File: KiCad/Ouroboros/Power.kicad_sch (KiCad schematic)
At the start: 8 parts, among them J2 Jack-DC, U1 Opamp_Quad, U3 LM78L05_TO92

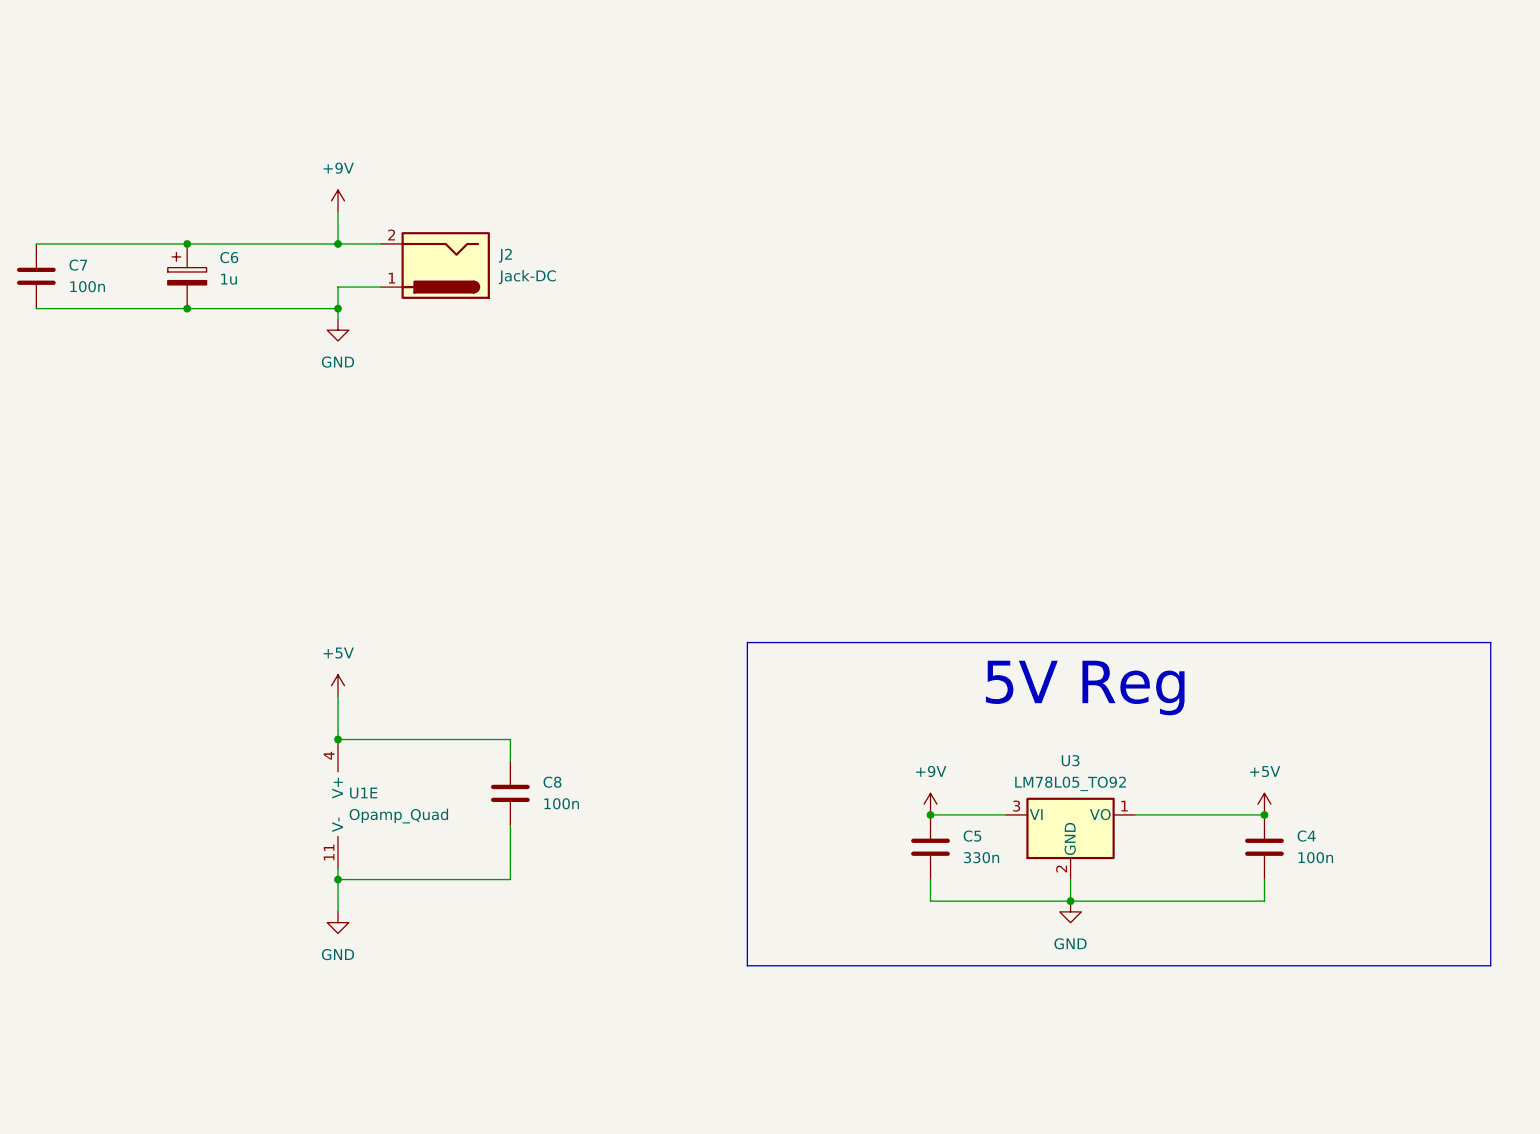
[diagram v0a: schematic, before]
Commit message: Updating schematic
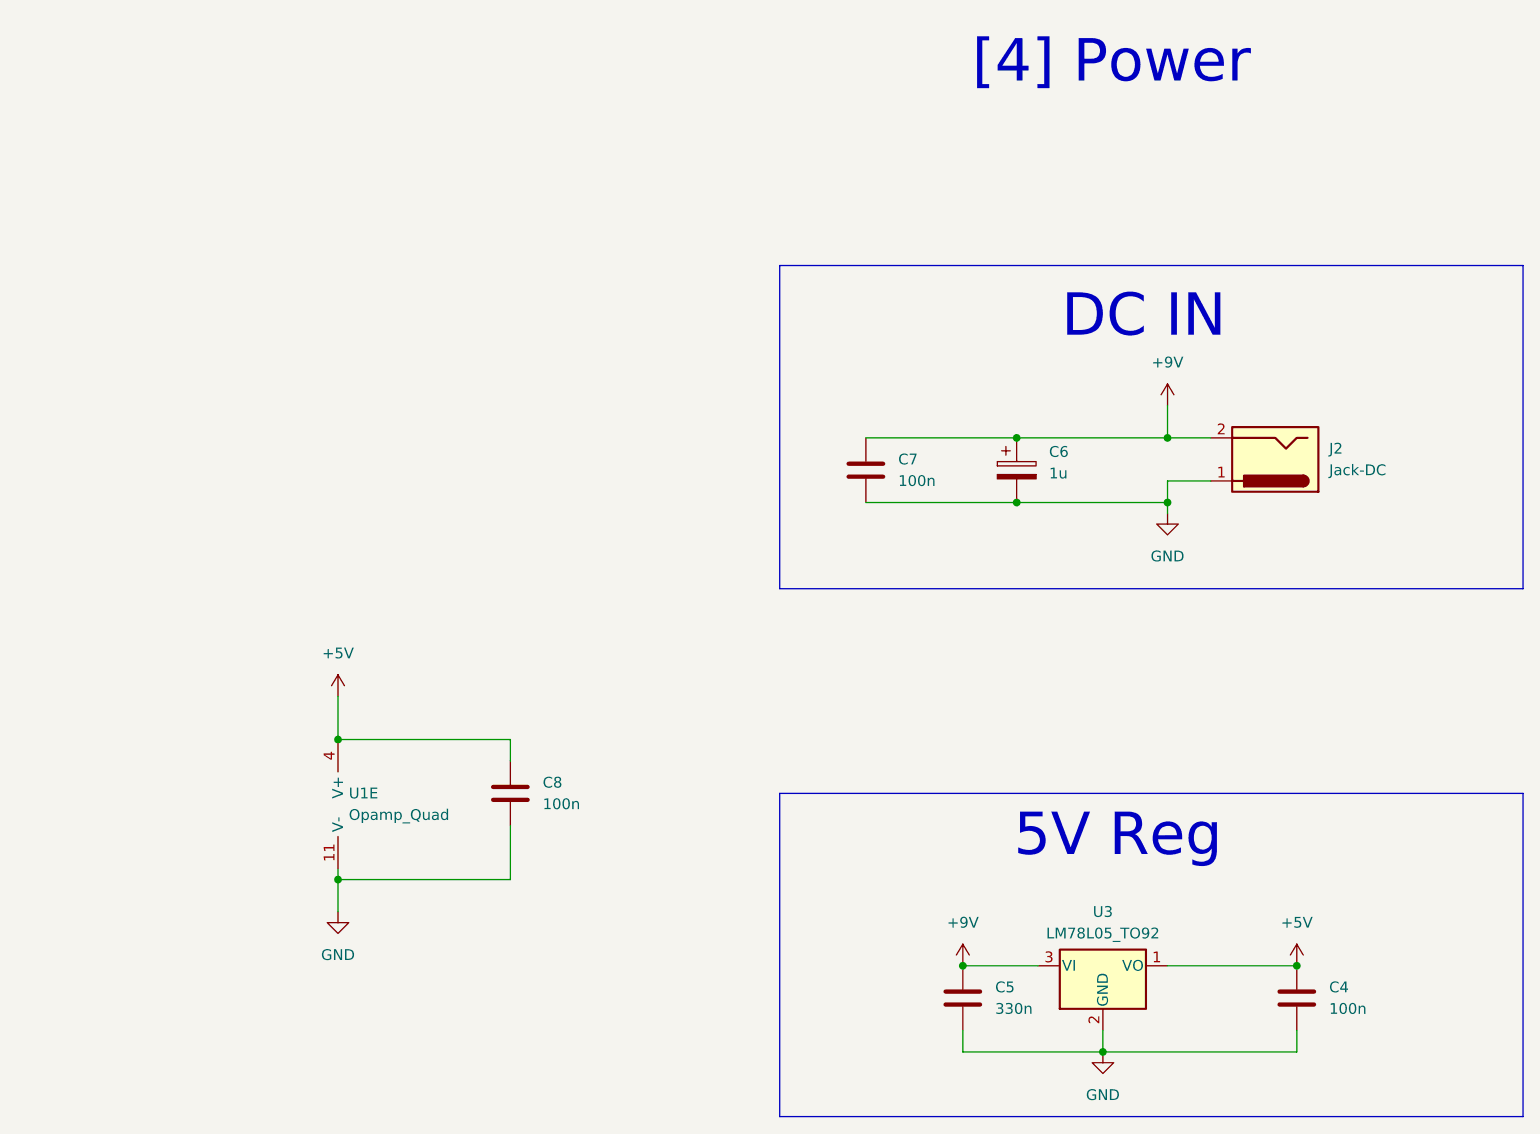
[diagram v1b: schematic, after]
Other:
- note added: "DC IN"
- note added: "[4] Power"
- moved on the sheet: C4, C5, C6, C7, J2, U3
